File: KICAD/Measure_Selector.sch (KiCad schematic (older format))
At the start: 2 parts

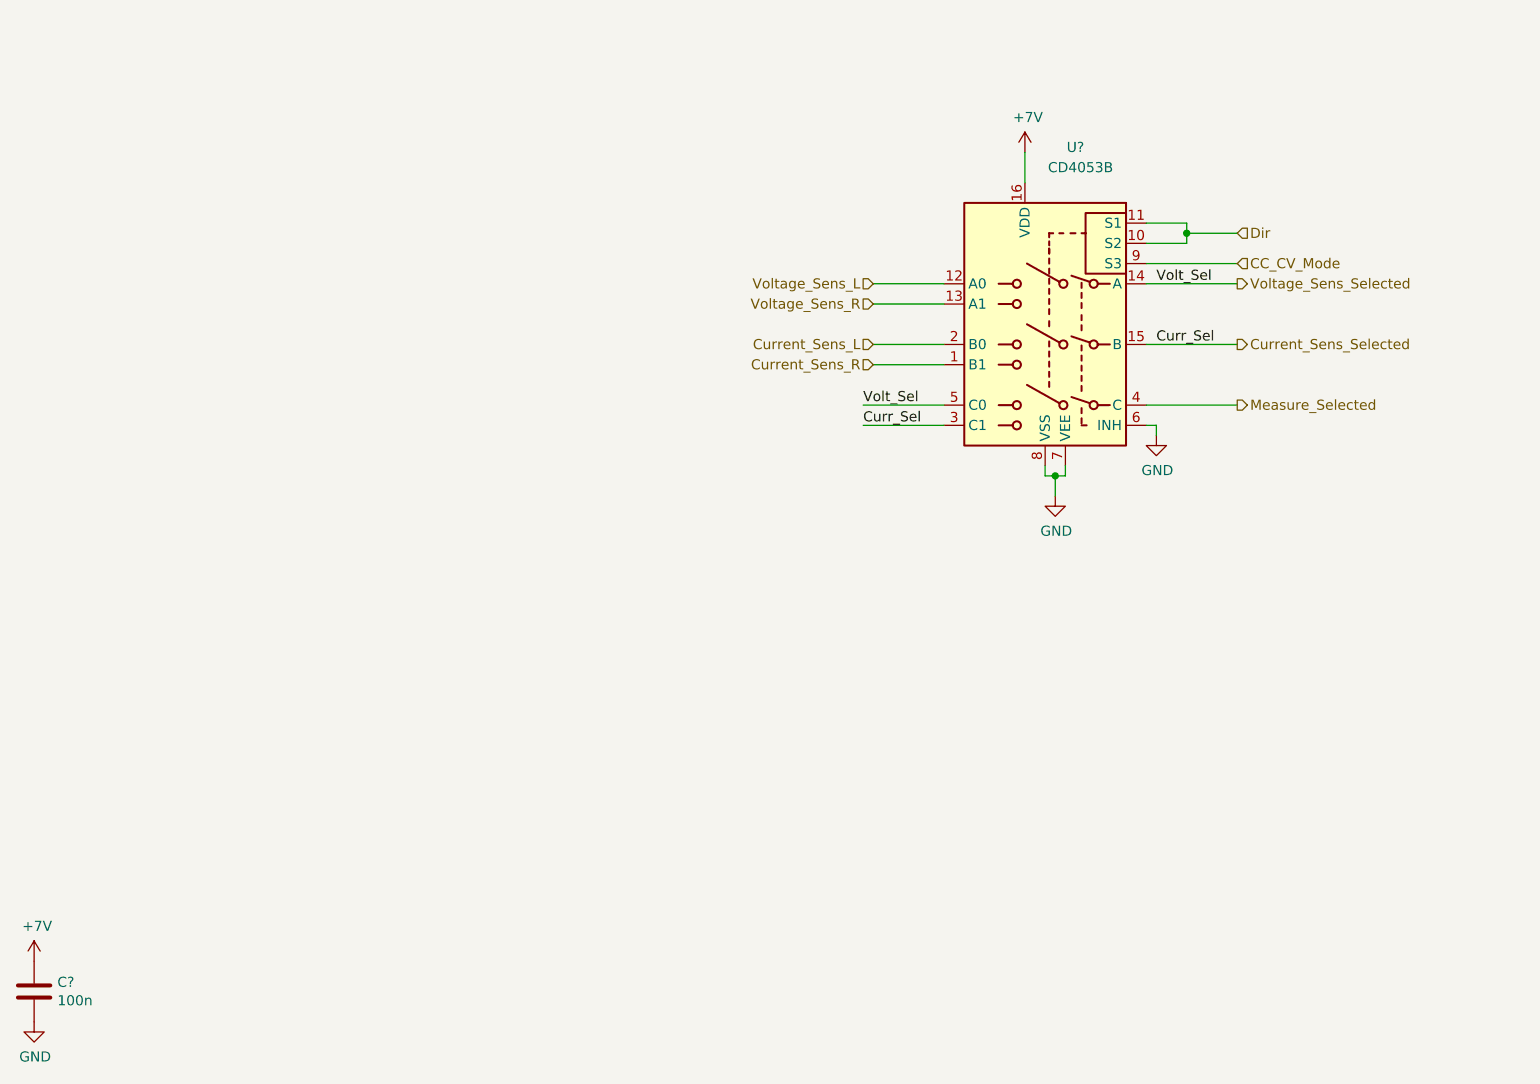
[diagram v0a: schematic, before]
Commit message: a ton of new stuff. V0.8
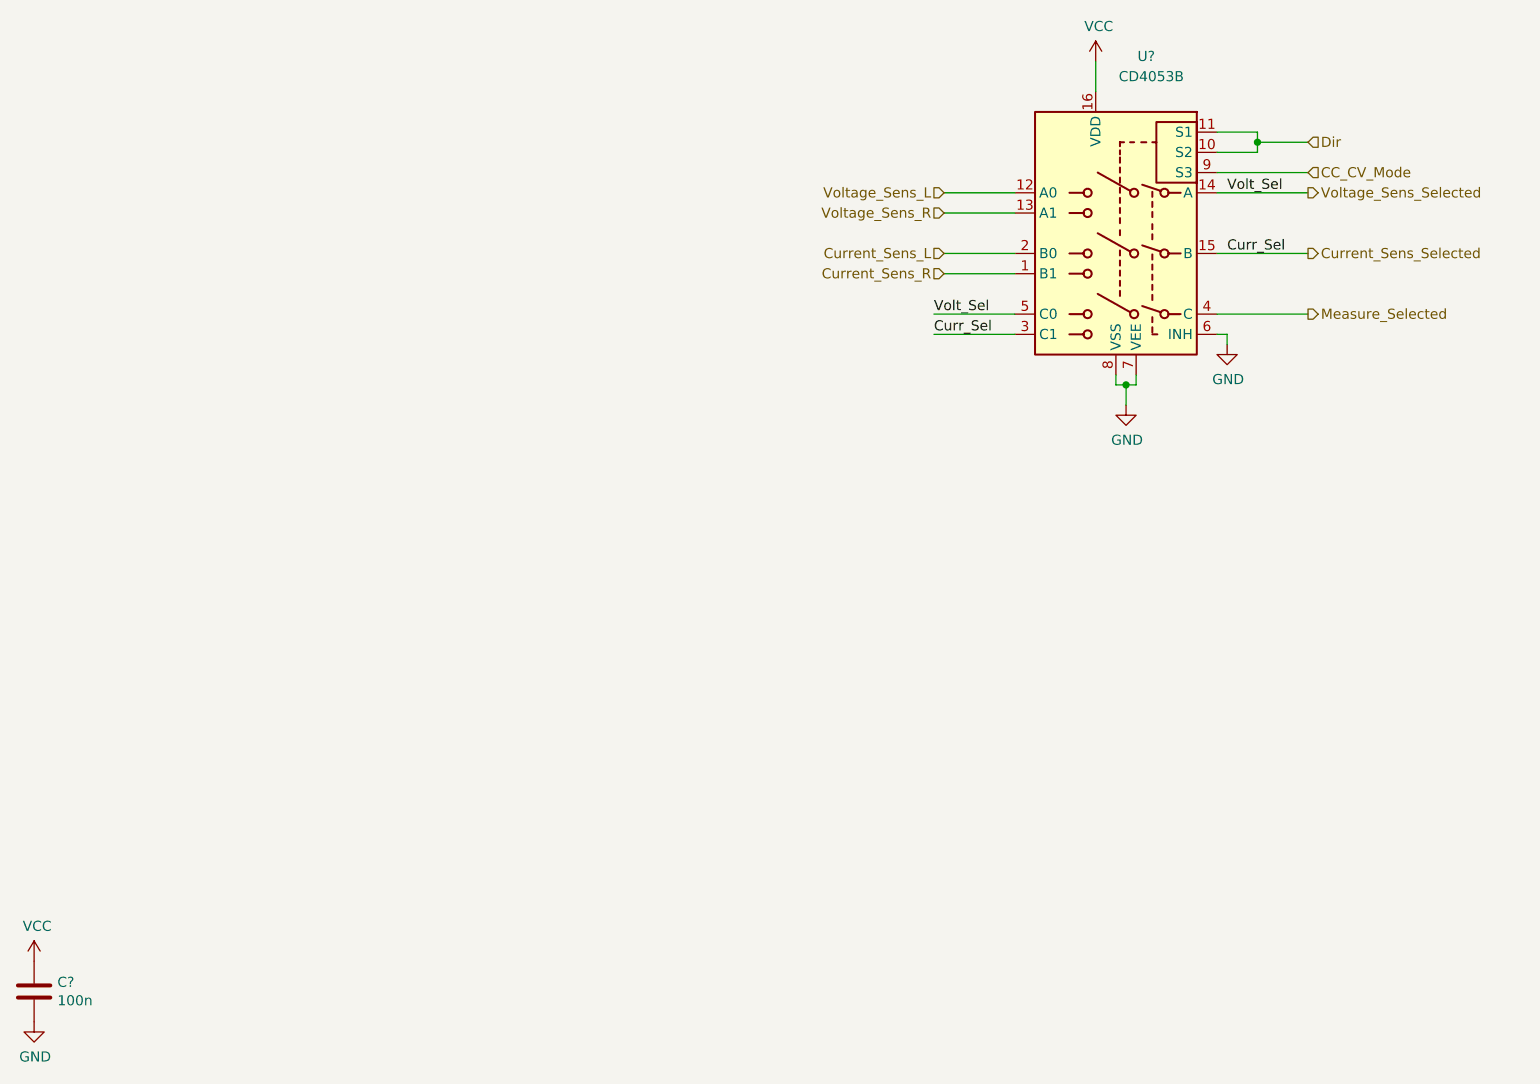
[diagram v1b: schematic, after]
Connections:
- net +7V renamed VCC
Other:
- moved on the sheet: U?
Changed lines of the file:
@@
 $Descr A4 11693 8268
 encoding utf-8
-Sheet 12 15
+Sheet 12 16
 Title "SESAME"
 Date "2021-08-03"
@@
 Comment4 ""
 $EndDescr
-Text HLabel 4900 3900 0    50   Input ~ 0
+Text HLabel 5250 3450 0    50   Input ~ 0
 Voltage_Sens_R
-Text HLabel 4900 4200 0    50   Input ~ 0
+Text HLabel 5250 3750 0    50   Input ~ 0
 Current_Sens_R
-Text HLabel 4900 3800 0    50   Input ~ 0
+Text HLabel 5250 3350 0    50   Input ~ 0
 Voltage_Sens_L
-Text HLabel 4900 4100 0    50   Input ~ 0
+Text HLabel 5250 3650 0    50   Input ~ 0
 Current_Sens_L
-Text HLabel 6700 3800 2    50   Output ~ 0
+Text HLabel 7050 3350 2    50   Output ~ 0
 Voltage_Sens_Selected
-Text HLabel 6700 4100 2    50   Output ~ 0
+Text HLabel 7050 3650 2    50   Output ~ 0
 Current_Sens_Selected
-Text HLabel 6700 3700 2    50   Input ~ 0
+Text HLabel 7050 3250 2    50   Input ~ 0
 CC_CV_Mode
-Text HLabel 6700 3550 2    50   Input ~ 0
+Text HLabel 7050 3100 2    50   Input ~ 0
 Dir
-Text HLabel 6700 4400 2    50   Output ~ 0
+Text HLabel 7050 3950 2    50   Output ~ 0
 Measure_Selected
 $Comp
 L sesame-fonctionnel-rescue:CD4053B-Analog_Switch U?
 U 1 1 610A09BD
-P 5750 4000
+P 6100 3550
 AR Path="/610A09BD" Ref="U?"  Part="1"
 AR Path="/60F421D1/610A09BD" Ref="U?"  Part="1"
-F 0 "U?" H 5600 4875 50  0000 C CNN
-F 1 "CD4053B" H 5575 4775 50  0000 C CNN
-F 2 "" H 5900 3250 50  0001 L CNN
-F 3 "http://www.ti.com/lit/ds/symlink/cd4052b.pdf" H 5730 4200 50  0001 C CNN
-	1    5750 4000
+F 0 "U?" H 5950 4425 50  0000 C CNN
+F 1 "CD4053B" H 5925 4325 50  0000 C CNN
+F 2 "" H 6250 2800 50  0001 L CNN
+F 3 "http://www.ti.com/lit/ds/symlink/cd4052b.pdf" H 6080 3750 50  0001 C CNN
+	1    6100 3550
 	-1   0    0    -1
 $EndComp
 Wire Wire Line
-	6250 3500 6450 3500
+	6600 3050 6800 3050
 Wire Wire Line
-	6450 3500 6450 3550
+	6800 3050 6800 3100
 Wire Wire Line
-	6450 3600 6250 3600
-Connection ~ 6450 3550
+	6800 3150 6600 3150
+Connection ~ 6800 3100
 Wire Wire Line
-	6450 3550 6450 3600
-Text Label 6300 3800 0    50   ~ 0
+	6800 3100 6800 3150
+Text Label 6650 3350 0    50   ~ 0
 Volt_Sel
-Text Label 6300 4100 0    50   ~ 0
+Text Label 6650 3650 0    50   ~ 0
 Curr_Sel
-Text Label 4850 4400 0    50   ~ 0
+Text Label 5200 3950 0    50   ~ 0
 Volt_Sel
-Text Label 4850 4500 0    50   ~ 0
+Text Label 5200 4050 0    50   ~ 0
 Curr_Sel
 $Comp
-L power:GND #PWR?
+L power:GND #PWR0161
 U 1 1 610E2D38
-P 6300 4550
-F 0 "#PWR?" H 6300 4300 50  0001 C CNN
-F 1 "GND" H 6305 4377 50  0000 C CNN
-F 2 "" H 6300 4550 50  0001 C CNN
-F 3 "" H 6300 4550 50  0001 C CNN
-	1    6300 4550
+P 6650 4100
+F 0 "#PWR0161" H 6650 3850 50  0001 C CNN
+F 1 "GND" H 6655 3927 50  0000 C CNN
+F 2 "" H 6650 4100 50  0001 C CNN
+F 3 "" H 6650 4100 50  0001 C CNN
+	1    6650 4100
 	1    0    0    -1
 $EndComp
 Wire Wire Line
-	6250 4500 6300 4500
+	6600 4050 6650 4050
 Wire Wire Line
-	6300 4500 6300 4550
+	6650 4050 6650 4100
 Wire Wire Line
-	5850 4700 5850 4750
+	6200 4250 6200 4300
 Wire Wire Line
-	5850 4750 5800 4750
+	6200 4300 6150 4300
 Wire Wire Line
-	5750 4750 5750 4700
+	6100 4300 6100 4250
 Wire Wire Line
-	5800 4750 5800 4850
-Connection ~ 5800 4750
+	6150 4300 6150 4400
+Connection ~ 6150 4300
 Wire Wire Line
-	5800 4750 5750 4750
+	6150 4300 6100 4300
 Wire Wire Line
-	6250 4400 6700 4400
+	6600 3950 7050 3950
 Wire Wire Line
-	6250 4100 6700 4100
+	6600 3650 7050 3650
 Wire Wire Line
-	6250 3800 6700 3800
+	6600 3350 7050 3350
 Wire Wire Line
-	6250 3700 6700 3700
+	6600 3250 7050 3250
 Wire Wire Line
-	6450 3550 6700 3550
+	6800 3100 7050 3100
 Wire Wire Line
-	5650 3150 5650 3300
+	6000 2700 6000 2850
 Wire Wire Line
-	5250 4400 4850 4400
+	5600 3950 5200 3950
 Wire Wire Line
-	5250 4500 4850 4500
+	5600 4050 5200 4050
 Wire Wire Line
-	5250 3800 4900 3800
+	5600 3350 5250 3350
 Wire Wire Line
-	4900 3900 5250 3900
+	5250 3450 5600 3450
 Wire Wire Line
-	5250 4100 4900 4100
+	5600 3650 5250 3650
 Wire Wire Line
-	4900 4200 5250 4200
+	5250 3750 5600 3750
 $Comp
-L power:GND #PWR?
+L power:GND #PWR0162
 U 1 1 610C24DF
-P 5800 4850
-F 0 "#PWR?" H 5800 4600 50  0001 C CNN
-F 1 "GND" H 5805 4677 50  0000 C CNN
-F 2 "" H 5800 4850 50  0001 C CNN
-F 3 "" H 5800 4850 50  0001 C CNN
-	1    5800 4850
+P 6150 4400
+F 0 "#PWR0162" H 6150 4150 50  0001 C CNN
+F 1 "GND" H 6155 4227 50  0000 C CNN
+F 2 "" H 6150 4400 50  0001 C CNN
+F 3 "" H 6150 4400 50  0001 C CNN
+	1    6150 4400
 	1    0    0    -1
 $EndComp
 $Comp
-L power:GND #PWR?
+L power:GND #PWR0163
 U 1 1 61122566
 P 750 7450
-F 0 "#PWR?" H 750 7200 50  0001 C CNN
+F 0 "#PWR0163" H 750 7200 50  0001 C CNN
 F 1 "GND" H 755 7277 50  0000 C CNN
 F 2 "" H 750 7450 50  0001 C CNN
@@
 $EndComp
 $Comp
-L Sesame:+7V #PWR?
-U 1 1 6128DF71
-P 5650 3150
-F 0 "#PWR?" H 5650 3000 50  0001 C CNN
-F 1 "+7V" H 5665 3323 50  0000 C CNN
-F 2 "" H 5650 3150 50  0001 C CNN
-F 3 "" H 5650 3150 50  0001 C CNN
-	1    5650 3150
-	1    0    0    -1
-$EndComp
-$Comp
-L Sesame:+7V #PWR?
-U 1 1 6128F549
+L power:VCC #PWR0164
+U 1 1 61547D97
 P 750 7150
-F 0 "#PWR?" H 750 7000 50  0001 C CNN
-F 1 "+7V" H 765 7323 50  0000 C CNN
+F 0 "#PWR0164" H 750 7000 50  0001 C CNN
+F 1 "VCC" H 765 7323 50  0000 C CNN
 F 2 "" H 750 7150 50  0001 C CNN
 F 3 "" H 750 7150 50  0001 C CNN
@@
 	1    0    0    -1
 $EndComp
+$Comp
+L power:VCC #PWR0165
+U 1 1 61549B3F
+P 6000 2700
+F 0 "#PWR0165" H 6000 2550 50  0001 C CNN
+F 1 "VCC" H 6015 2873 50  0000 C CNN
+F 2 "" H 6000 2700 50  0001 C CNN
+F 3 "" H 6000 2700 50  0001 C CNN
+	1    6000 2700
+	1    0    0    -1
+$EndComp
